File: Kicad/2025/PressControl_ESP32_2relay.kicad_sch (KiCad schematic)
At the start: 35 parts, among them J1 Conn_01x08_Pin, J10 Conn_01x08_Socket, J11 Conn_01x08_Socket, J12 SIP_01, J13 SIP_01, J14 Conn_01x08_Pin, J15 Conn_01x08_Socket, J16 Conn_01x08_Pin, J2 Conn_01x08_Socket, J3 Conn_01x08_Pin, J8 Conn_01x08_Socket, J9 Conn_01x08_Pin, K1 RELAY_1RT, K2 RELAY_1RT, K3 Relayx2_Module, P1 Pump, P2 Press_Control, SW2 startPControl, SW3 startPControl, U1 ESP32-WROOM-32b

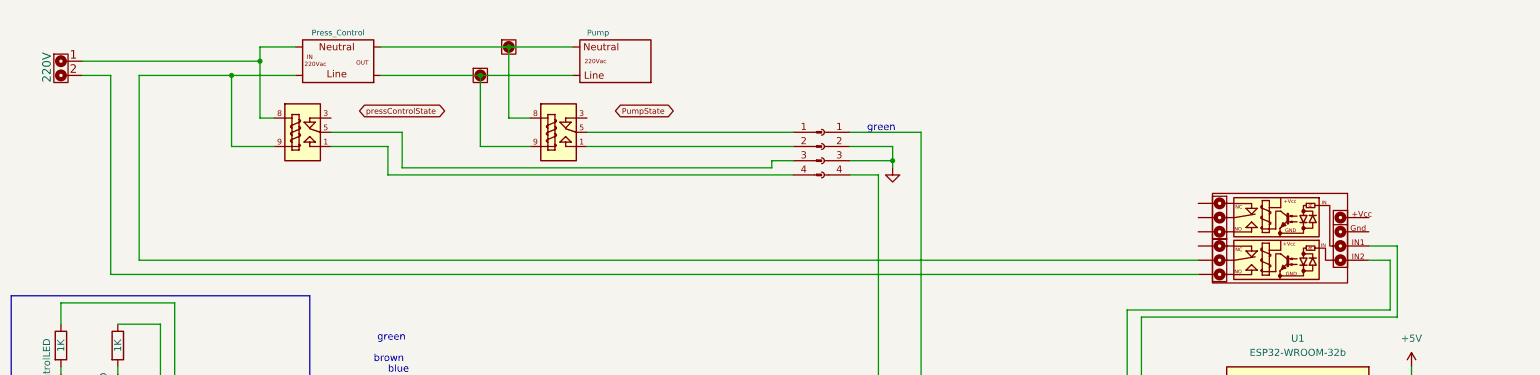
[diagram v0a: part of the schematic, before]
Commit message: update kicad
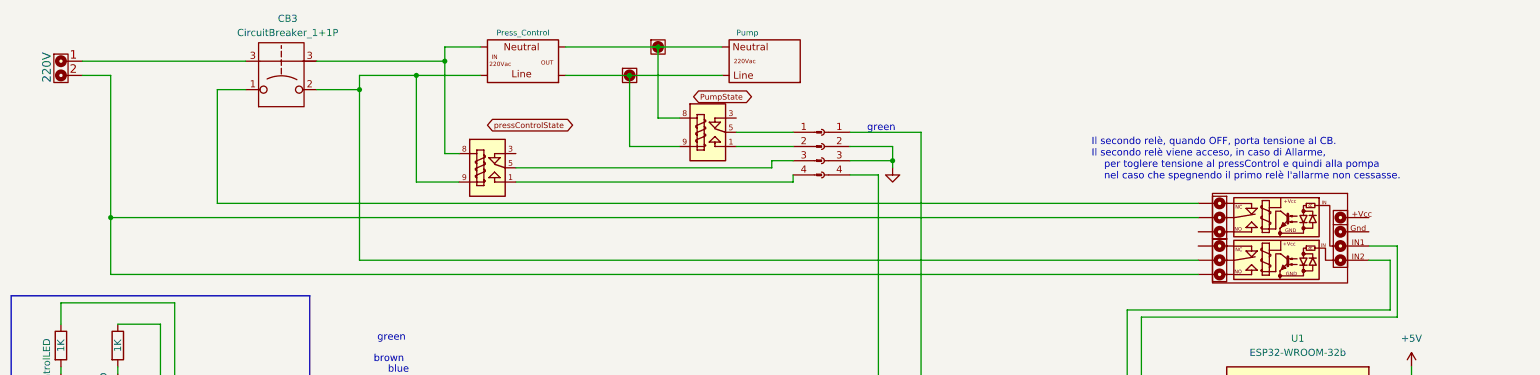
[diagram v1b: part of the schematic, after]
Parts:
- added CB3: CircuitBreaker_1+1P, symbol lnConnectors:CircuitBreaker_1+1P
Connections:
- net at J?.2, K3.3 (IN1): now also K3.2 (GND)
- net at K3.1 (VCC): now also CB3.1
- net at K3.3 (IN1): now also U1.28 (G.17)
- new net: CB3.3, J?.1
- new net: CB3.3, K1.8, P2.~ (2)
- new net: CB3.2, K1.9, K3.2 (GND), P2.~ (2)
- now unconnected: K3.2 (GND)
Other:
- note added: "Il secondo relè, quando OFF, porta tensione al CB. Il secondo relè viene acceso, in caso di Allarme, per toglere tensione al pressControl e quindi alla pompa nel caso che spegnendo il primo relè l'allarme non cessasse."

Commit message: kicad schematic changes
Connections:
- net at K3.1: now also CB3.1
- net at K3.3: now also U1.28 (G.17)
- new net: J?.2, K3.2, K3.3
- now unconnected: K3.2 (GND)
